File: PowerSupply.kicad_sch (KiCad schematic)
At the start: 35 parts, among them J1 S2B-ZRLFSN, J2 Native USB, J3 Native USB, U1 CH340E, U2 NCP1117-5.0_SOT223, U3 TPS2115ADRBR, U4 ld39150dt33-r, U5 USBLC6-2SC6, U6 USBLC6-2SC6

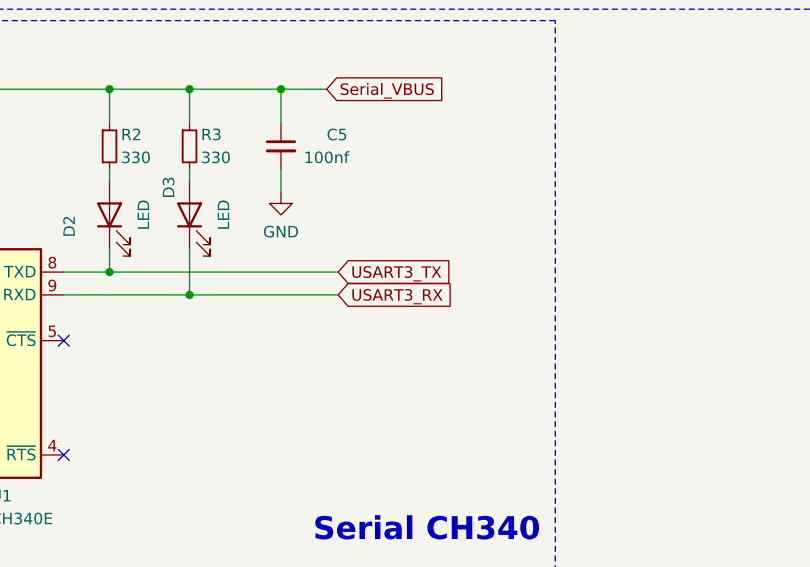
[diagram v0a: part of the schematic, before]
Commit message: update
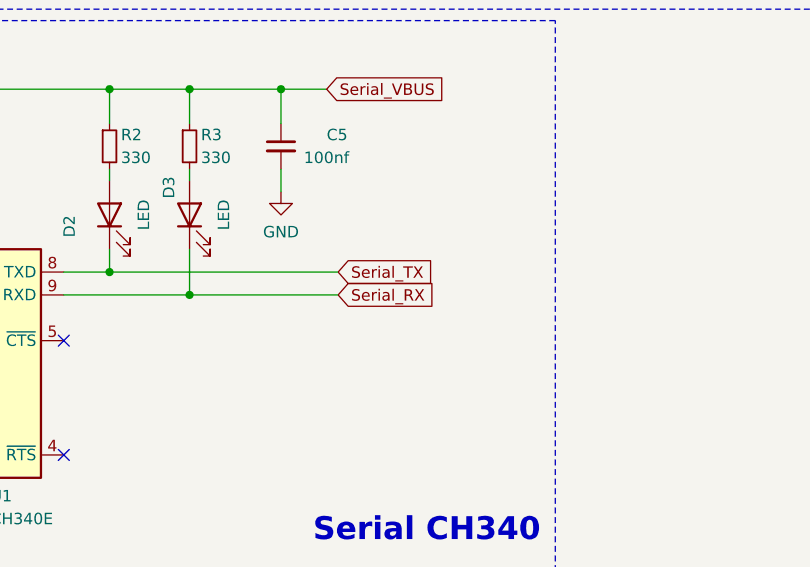
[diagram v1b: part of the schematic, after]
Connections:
- net USART3_RX renamed Serial_RX
- net USART3_TX renamed Serial_TX
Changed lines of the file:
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@@
+		)
+	)
+	(global_label "Serial_TX"
+		(shape input)
+		(at 86.36 162.56 0)
+		(effects
+			(font
+				(size 1.27 1.27)
+			)
+			(justify left)
+		)
+		(property "Intersheetrefs" "${INTERSHEET_REFS}"
+			(at 86.36 162.56 0)
+			(effects
+				(font
+					(size 1.27 1.27)
+				)
+				(hide yes)
+			)
 		)
 	)
@@
 		)
 	)
+	(global_label "Serial_RX"
+		(shape input)
+		(at 86.36 165.1 0)
+		(effects
+			(font
+				(size 1.27 1.27)
+			)
+			(justify left)
+		)
+		(property "Intersheetrefs" "${INTERSHEET_REFS}"
+			(at 86.36 165.1 0)
+			(effects
+				(font
+					(size 1.27 1.27)
+				)
+				(hide yes)
+			)
+		)
+	)
 	(global_label "C_Serial_D+"
 		(shape input)
@@
 		)
 	)
-	(global_label "USART3_TX"
-		(shape input)
-		(at 86.36 162.56 0)
-		(fields_autoplaced yes)
-		(effects
-			(font
-				(size 1.27 1.27)
-			)
-			(justify left)
-		)
-		(property "Intersheetrefs" "${INTERSHEET_REFS}"
-			(at 99.5656 162.56 0)
-			(effects
-				(font
-					(size 1.27 1.27)
-				)
-				(justify left)
-				(hide yes)
-			)
-		)
-	)
 	(global_label "Serial_D-"
 		(shape input)
@@
 			(effects
 				(font
-					(size 1.27 1.27)
-				)
-				(justify left)
-				(hide yes)
-			)
-		)
-	)
-	(global_label "USART3_RX"
-		(shape input)
-		(at 86.36 165.1 0)
-		(fields_autoplaced yes)
-		(effects
-			(font
-				(size 1.27 1.27)
-			)
-			(justify left)
-		)
-		(property "Intersheetrefs" "${INTERSHEET_REFS}"
-			(at 99.868 165.1 0)
-			(effects
-				(font

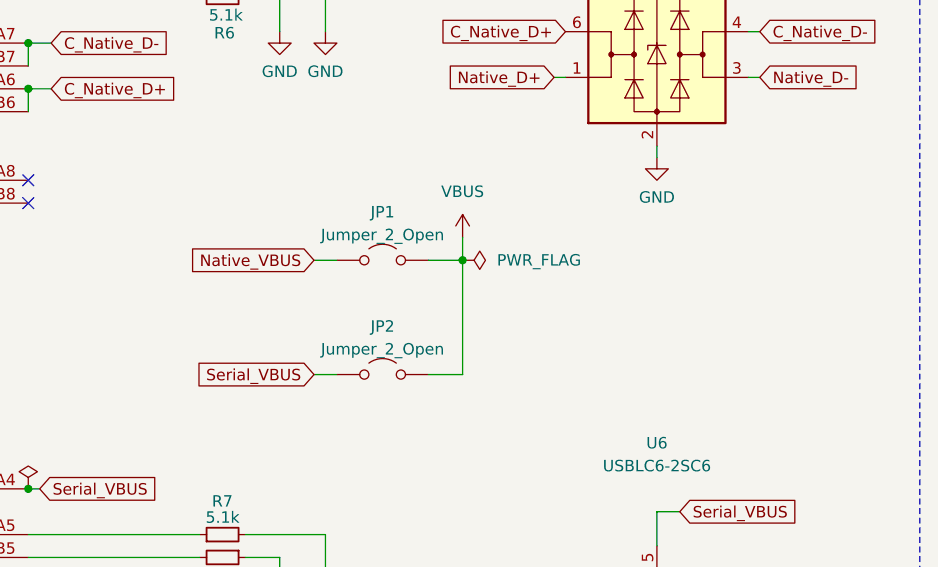
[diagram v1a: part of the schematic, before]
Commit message: update
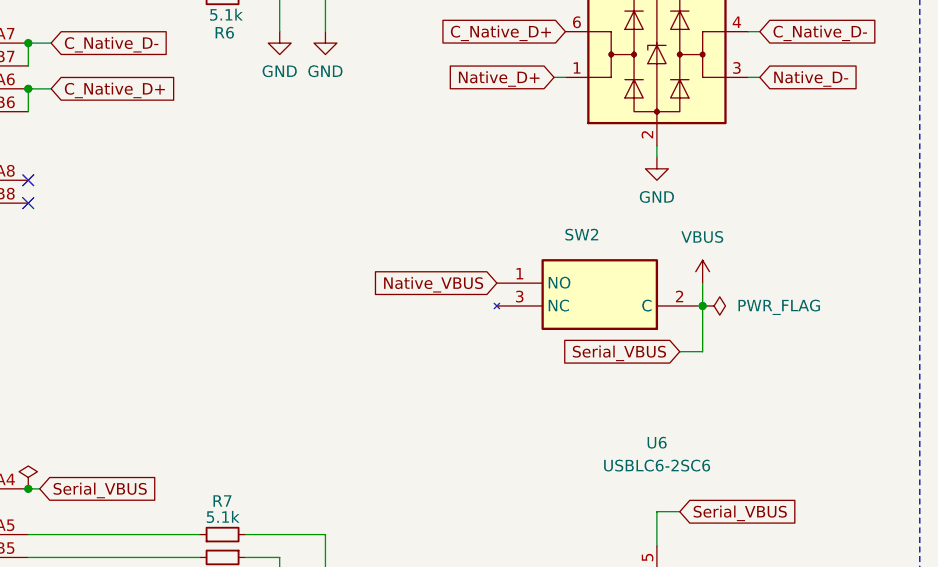
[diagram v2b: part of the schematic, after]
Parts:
- removed JP1, JP2: Jumper_2_Open, Connector_PinHeader_2.54mm:PinHeader_1x02_P2.54mm_Vertical, symbol Jumper:Jumper_2_Open
- added SW2: SSSS213000, mylib:SSSS213000, symbol SSSS213000:SSSS213000
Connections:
- net Serial_VBUS is gone; now on net VBUS: C5.1, J3.A4 (VBUS), J3.A9 (VBUS), J3.B4 (VBUS), J3.B9 (VBUS), R2.1, R3.1, U1.7 (VCC), U6.5 (VBUS)
- net Native_VBUS: now also SW2.1 (NO)
- net VBUS: now also SW2.2 (C)
